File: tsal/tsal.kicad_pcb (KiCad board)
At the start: 2 copper layers, 34.3 x 52.1 mm, 20 parts, among them P1 TS+ (PreAIR), P2 TS-, P3 CONN_01X01, P4 CONN_01X01, P5 TS+ (PostAIR), P6 CONN_01X01, P7 CONN_01X01, U1 V36SE12004NRFA, U2 TL431

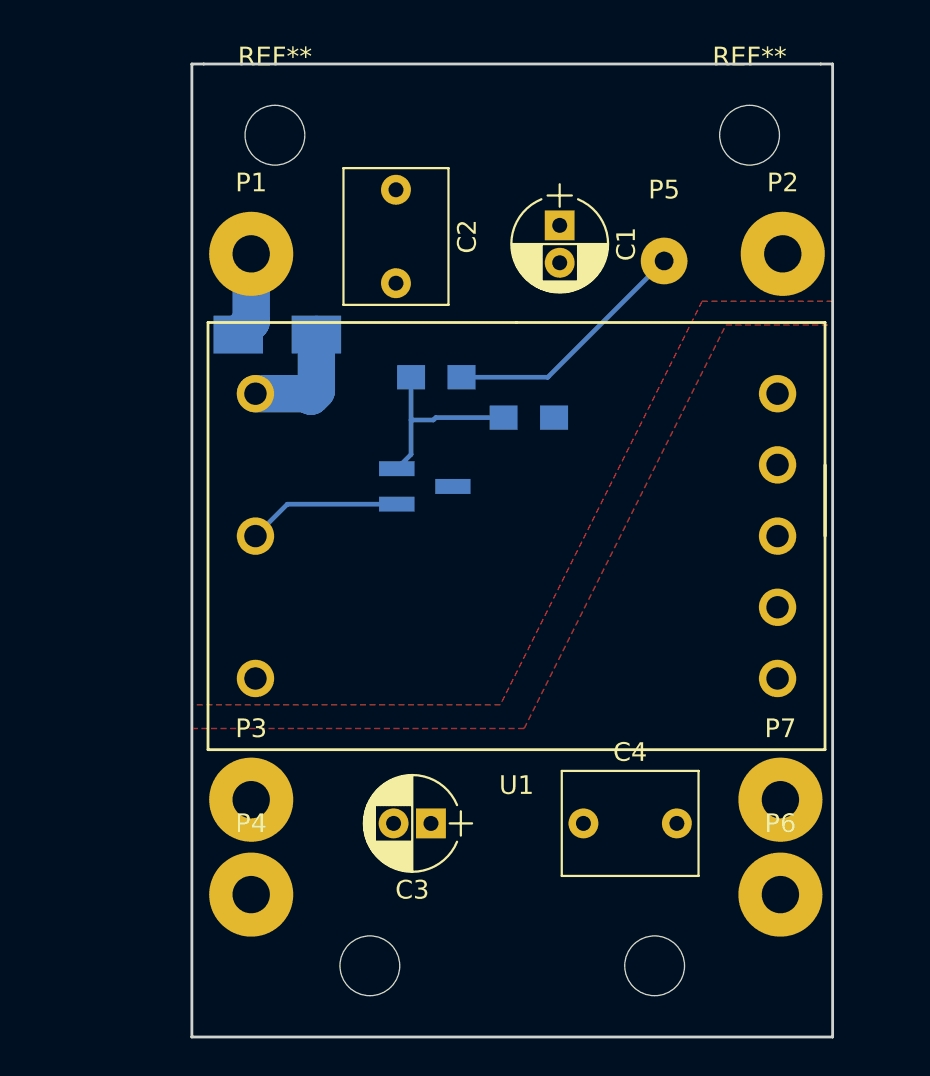
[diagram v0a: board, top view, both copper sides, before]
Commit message: TSAL board layout
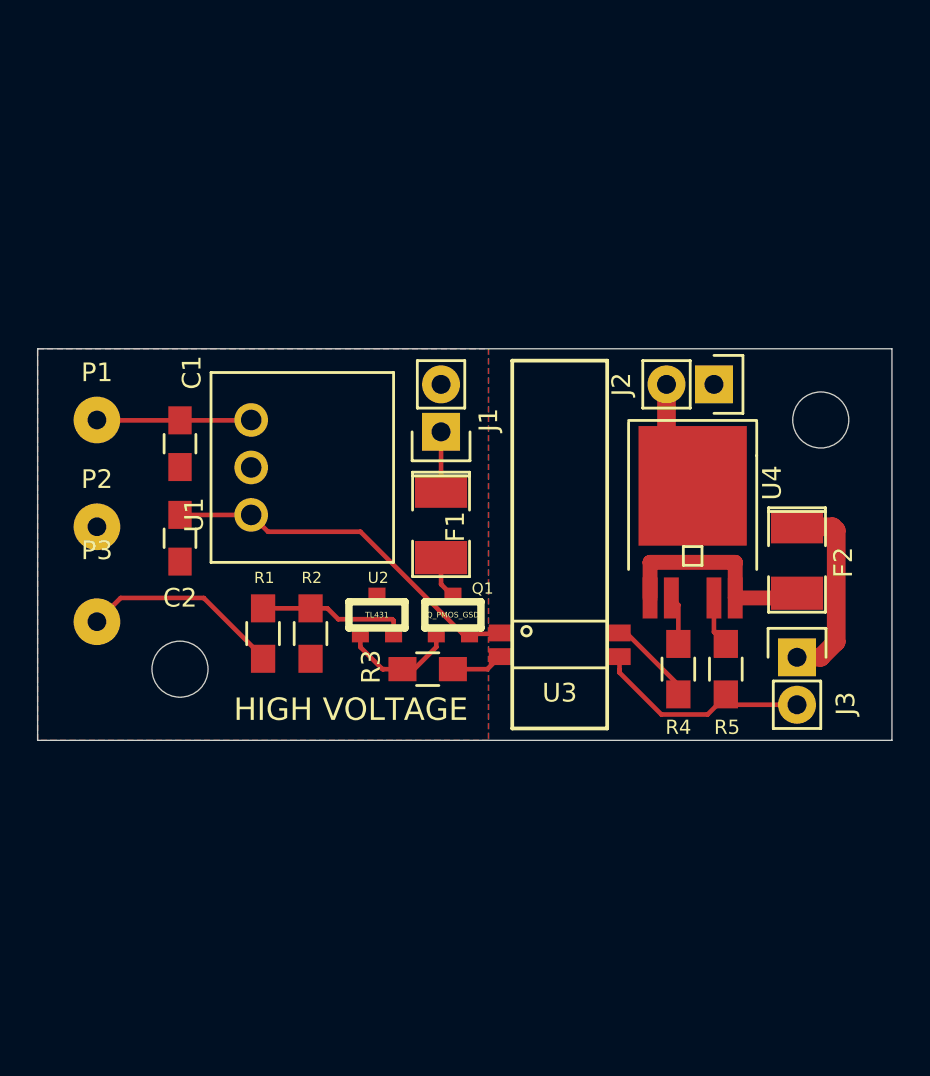
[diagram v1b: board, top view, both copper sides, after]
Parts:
- removed C3: 10u, Capacitors_ThroughHole:CP_Radial_D5.0mm_P2.00mm
- removed C4: 1u, Capacitors_ThroughHole:C_Rect_L7.2mm_W5.5mm_P5.00mm_FKS2_FKP2_MKS2_MKP2
- removed P4, P6, P7: CONN_01X01, Wire_Pads:SolderWirePad_single_2mmDrill
- removed P5: TS+ (PostAIR), Wire_Pads:SolderWirePad_single_1mmDrill
- removed REF** (x4): MountingHole_3.2mm_M3, Mounting_Holes:MountingHole_3.2mm_M3
- added F2: 3A, SMD_Packages:SMD-1210_Pol, F.Cu at (132.1, 92.6)
- added G***: LOGO, UNCAMotorsports:UNCA Logo, B.Cu at (119.4, 92.1)
- added J1: Indicator, Pin_Headers:Pin_Header_Straight_1x02, F.Cu at (113.0, 85.7)
- added J2: GLV, Pin_Headers:Pin_Header_Straight_1x02, F.Cu at (127.6, 83.2)
- added J3: TSAL, Pin_Headers:Pin_Header_Straight_1x02, F.Cu at (132.1, 97.8)
- added MK1: Mounting_Hole, Mounting_Holes:MountingHole_3mm, F.Cu at (99.1, 98.4)
- added MK3: Mounting_Hole, Mounting_Holes:MountingHole_3mm, F.Cu at (133.3, 85.1)
- added Q1: Q_PMOS_GSD, UNCAMotorsports:SOT23-3, F.Cu at (113.7, 95.5)
- added R3: 1.2k, Resistors_SMD:R_0805_HandSoldering, F.Cu at (112.3, 98.4)
- added R4: 0R, Resistors_SMD:R_0805_HandSoldering, F.Cu at (125.7, 98.4)
- added R5: 1k, Resistors_SMD:R_0805_HandSoldering, F.Cu at (128.3, 98.4)
- added U3: TCMT1103, UNCAMotorsports:SSOP-4, F.Cu at (119.4, 97.2)
- added U4: BTS6133D, UNCAMotorsports:TO-252-5, F.Cu at (126.5, 88.6)
- C1: value 10u -> 10uF; footprint Capacitors_ThroughHole:CP_Radial_D5.0mm_P2.00mm -> Capacitors_SMD:C_0805_HandSoldering
- C2: value 1u -> 10uF; footprint Capacitors_ThroughHole:C_Rect_L7.2mm_W5.5mm_P5.00mm_FKS2_FKP2_MKS2_MKP2 -> Capacitors_SMD:C_0805_HandSoldering
- F1: value Fuse -> 3A; footprint Fuse_Holders_and_Fuses:Fuse_SMD1206_HandSoldering -> SMD_Packages:SMD-1210_Pol; moved to F.Cu
- P1, P2: footprint Wire_Pads:SolderWirePad_single_2mmDrill -> Wire_Pads:SolderWirePad_single_1mmDrill
- P3: value CONN_01X01 -> TS+ (PostAIR); footprint Wire_Pads:SolderWirePad_single_2mmDrill -> Wire_Pads:SolderWirePad_single_1mmDrill
- R1, R2: moved to F.Cu
- U1: value V36SE12004NRFA -> V7812W-500; footprint UNCAMotorsports:V36SE12004NRFA -> UNCAMotorsports:V78W-500
- U2: footprint TO_SOT_Packages_SMD:SOT-23_Handsoldering -> UNCAMotorsports:SOT23-3; moved to F.Cu
- moved P2 39.5 mm to (94.6, 90.8)
- moved C1 23.4 mm to (99.1, 86.4)
- moved C2 21.9 mm to (99.1, 91.4)
- moved R1 16.6 mm to (103.5, 96.5), turned to 90 degrees
- moved R2 16.4 mm to (106.0, 96.5), turned to 270 degrees
- moved U1 14.7 mm to (102.9, 87.6), turned to 90 degrees
- moved F1 13.4 mm to (113.0, 90.7), turned to 270 degrees
- moved P3 12.6 mm to (94.6, 95.9)
- moved P1 12.1 mm to (94.6, 85.1)
- moved U2 7.34 mm to (109.6, 95.5), turned to 180 degrees
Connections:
- C1 pad 2: GND -> GNDA
- C2 pad 1: Net-(C1-Pad1) -> Net-(C2-Pad1)
- C2 pad 2: GND -> GNDA
- F1 pad 1: Net-(C1-Pad1) -> Net-(F1-Pad1)
- P1 pad 1: Net-(F1-Pad2) -> Net-(C1-Pad1)
- P2 pad 1: GND -> GNDA
- P3 pad 1: Net-(C3-Pad1) -> Net-(P3-Pad1)
- R1 pad 1: Net-(P5-Pad1) -> Net-(P3-Pad1)
- R2 pad 2: GND -> GNDA
- U1 pad 2: Net-(U1-Pad2) -> GNDA
- U1 pad 3: GND -> Net-(C2-Pad1)
- U2 pad 1: Net-(U1-Pad2) -> Net-(Q1-Pad1)
- U2 pad 3: GND -> GNDA
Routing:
- net Net-(C2-Pad1): track 0.00 -> 19.8 mm
- net Net-(P5-Pad1): track 13.4 -> 0.00 mm
- net GND: track 0.00 -> 12.2 mm
- net Net-(F2-Pad2): track 0.00 -> 11.0 mm
- net Net-(P3-Pad1): track 0.00 -> 10.8 mm
- net Net-(F2-Pad1): track 0.00 -> 10.6 mm
- net Net-(U1-Pad2): track 8.27 -> 0.00 mm
- net Net-(J2-Pad2): track 0.00 -> 8.21 mm
- net Net-(Q1-Pad1): track 0.00 -> 6.46 mm
- net Net-(R4-Pad1): track 0.00 -> 4.81 mm
- net Net-(R4-Pad2): track 0.00 -> 3.32 mm
- net Net-(F1-Pad1): track 0.00 -> 3.18 mm
- net Net-(R3-Pad1): track 0.00 -> 2.79 mm
- net Net-(R5-Pad1): track 0.00 -> 2.72 mm
- net Net-(F1-Pad2): track 4.61 -> 2.33 mm
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- added copper zone on B.Cu, net GNDA
- added copper zone on F.Cu, net GNDA
- removed copper zone on B.Cu, net GND
- removed copper zone on F.Cu, net Net-(C1-Pad1)
- removed copper zone on F.Cu, net Net-(C3-Pad1)
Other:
- board size 34.3 x 52.1 mm -> 45.7 x 21 mm
- net class Default: via_dia 0.8 -> 0.6
- rule pad_to_mask_clearance: 0.2 -> 0
- board text added: "Designed By Paul Guenette May 10, 2017 Rev 1"
- board text added: "HIGH VOLTAGE"
